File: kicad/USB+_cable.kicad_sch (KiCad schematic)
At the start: 6 parts, among them J1601 USB_C_Receptacle, J1602 USB_C_Receptacle, J1603 USB3.1_full_cable

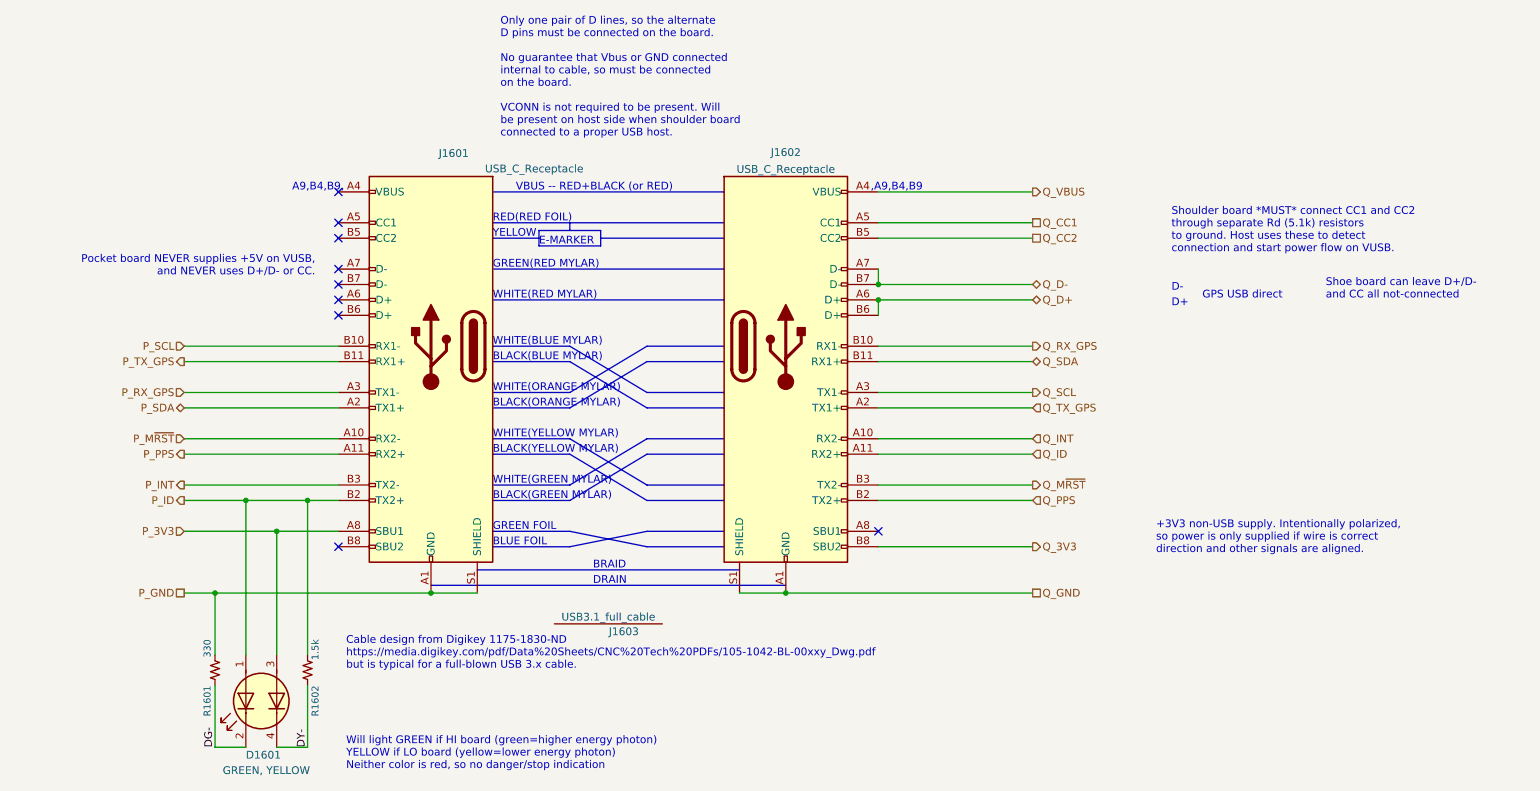
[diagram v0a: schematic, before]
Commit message: Added a NC to the board
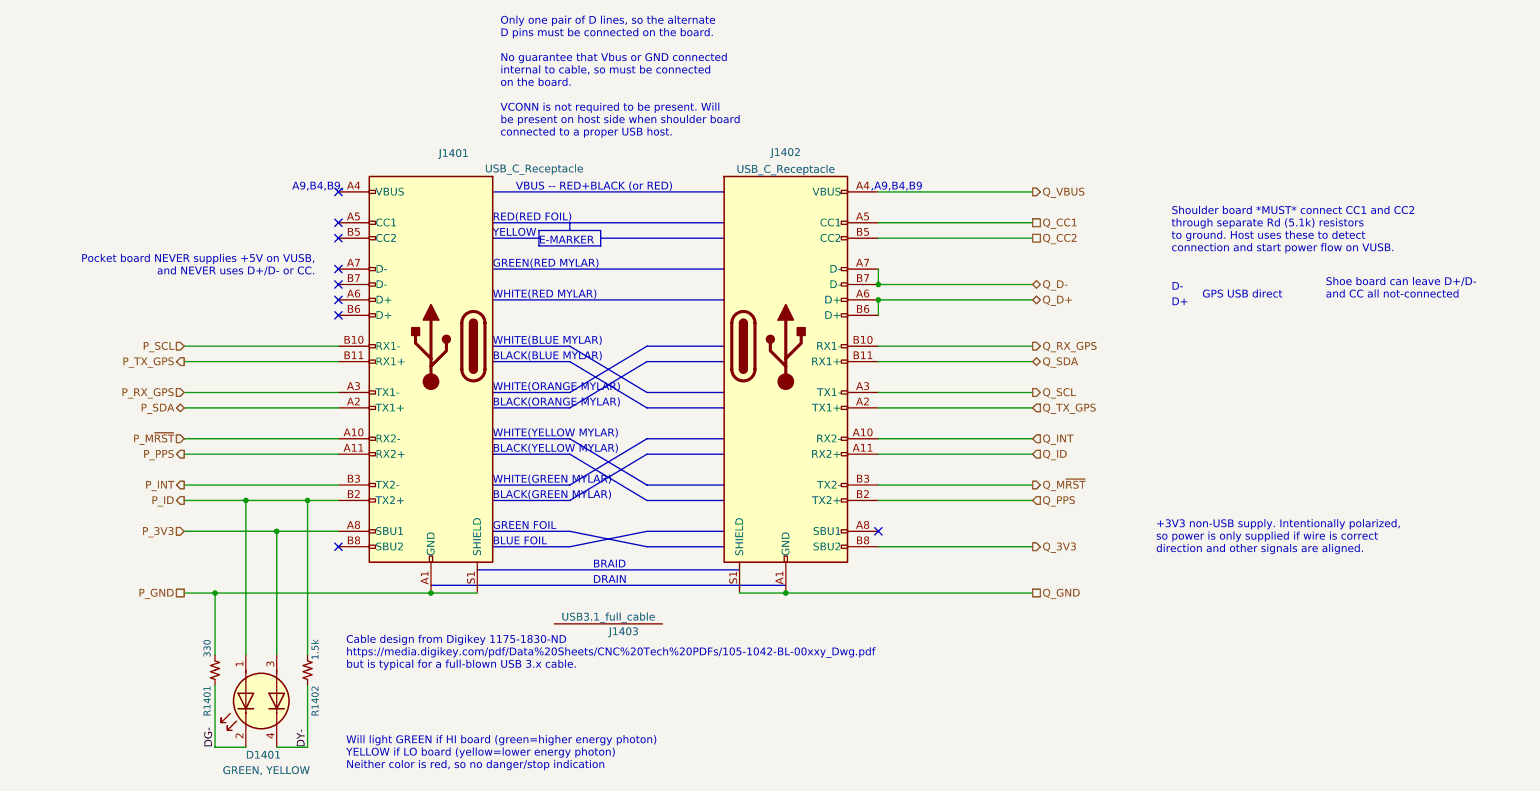
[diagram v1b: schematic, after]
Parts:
- renumbered D1601 to D1401, J1601 to J1401, J1602 to J1402, J1603 to J1403, R1601 to R1401, R1602 to R1402
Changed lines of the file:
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@@
   (symbol (lib_id "Connector:USB_C_Receptacle") (at 154.94 88.9 0) (mirror y)
     (in_bom yes) (on_board yes)
-    (property "Reference" "J1601" (id 0) (at 156.21 57.15 0)
+    (property "Reference" "J1401" (id 0) (at 156.21 57.15 0)
       (effects (font (size 1.27 1.27)) (justify right))
     )
@@
   (symbol (lib_id "Device:LED_Dual_AKAK") (at 127 147.32 90) (mirror x)
     (in_bom yes) (on_board yes)
-    (property "Reference" "D1601" (id 0) (at 124.46 156.21 90)
+    (property "Reference" "D1401" (id 0) (at 124.46 156.21 90)
       (effects (font (size 1.27 1.27)) (justify right))
     )
@@
   (symbol (lib_id "KwanSystems:RESISTOR") (at 119.38 142.24 90)
     (in_bom yes) (on_board yes)
-    (property "Reference" "R1601" (id 0) (at 118.11 144.78 0)
+    (property "Reference" "R1401" (id 0) (at 118.11 144.78 0)
       (effects (font (size 1.143 1.143)) (justify right))
     )
@@
   (symbol (lib_id "Connector:USB_C_Receptacle") (at 213.36 88.9 0)
     (in_bom yes) (on_board yes) (fields_autoplaced)
-    (property "Reference" "J1602" (id 0) (at 213.36 56.9935 0))
+    (property "Reference" "J1402" (id 0) (at 213.36 56.9935 0))
     (property "Value" "USB_C_Receptacle" (id 1) (at 213.36 59.7686 0))
     (property "Footprint" "KwanSystems:USB_C_Amphenol_MidMount" (id 2) (at 217.17 88.9 0)
@@
   (symbol (lib_id "KwanSystems:USB3.1_full_cable") (at 184.15 133.35 0)
     (in_bom yes) (on_board no)
-    (property "Reference" "J1603" (id 0) (at 186.69 135.89 0))
+    (property "Reference" "J1403" (id 0) (at 186.69 135.89 0))
     (property "Value" "USB3.1_full_cable" (id 1) (at 184.15 133.4794 0))
     (property "Footprint" "" (id 2) (at 184.15 133.35 0)
@@
   (symbol (lib_id "KwanSystems:RESISTOR") (at 134.62 142.24 90)
     (in_bom yes) (on_board yes)
-    (property "Reference" "R1602" (id 0) (at 135.89 144.78 0)
+    (property "Reference" "R1402" (id 0) (at 135.89 144.78 0)
       (effects (font (size 1.143 1.143)) (justify right))
     )
